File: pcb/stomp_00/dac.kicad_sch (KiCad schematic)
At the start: 6 parts, among them J4 Headphones, U9 SGTL5000XNAA3

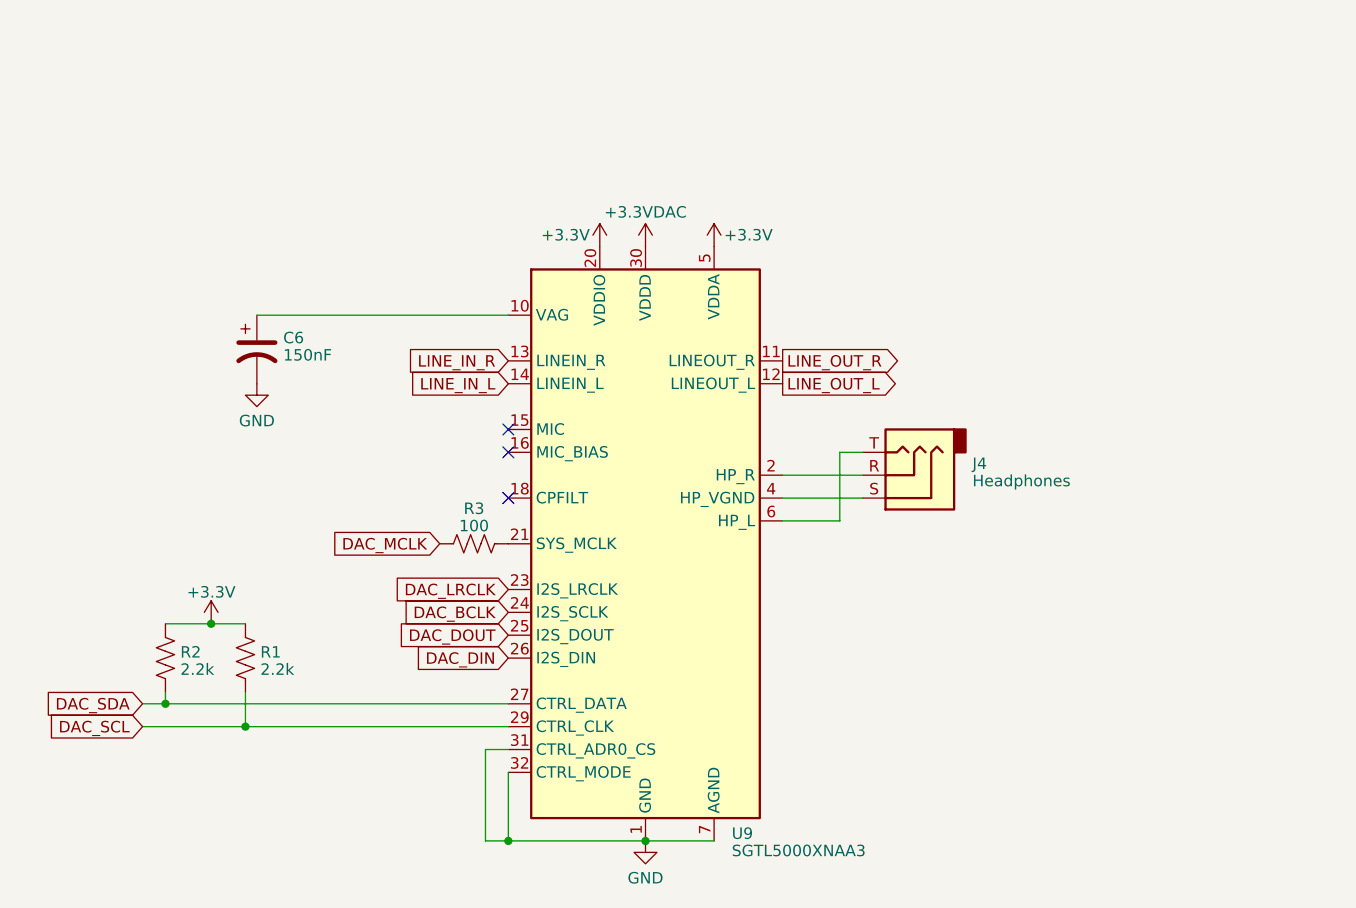
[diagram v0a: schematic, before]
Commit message: more input stage faffing
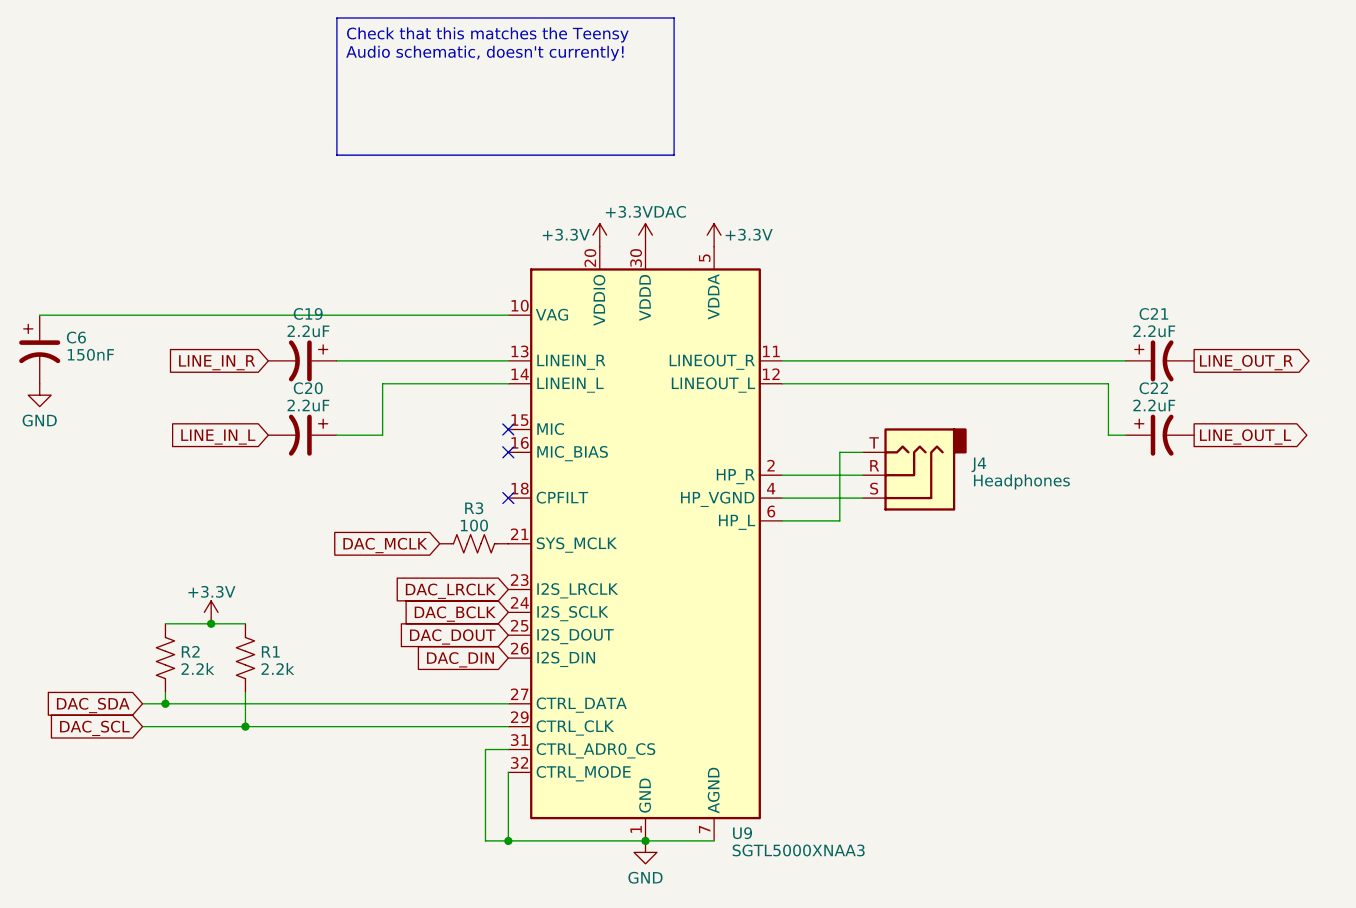
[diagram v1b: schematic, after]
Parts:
- added C19, C20, C21, C22: 2.2uF, symbol Device:C_Polarized_US
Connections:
- net LINE_IN_L: now also C20.2; no longer U9.14 (LINEIN_L)
- net LINE_IN_R: now also C19.2; no longer U9.13 (LINEIN_R)
- net LINE_OUT_L: now also C22.2; no longer U9.12 (LINEOUT_L)
- net LINE_OUT_R: now also C21.2; no longer U9.11 (LINEOUT_R)
- new net: C21.1, U9.11 (LINEOUT_R)
- new net: C22.1, U9.12 (LINEOUT_L)
- new net: C19.1, U9.13 (LINEIN_R)
- new net: C20.1, U9.14 (LINEIN_L)
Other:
- moved on the sheet: C6
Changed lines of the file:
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@@
+    (stroke (width 0) (type default))
+  )
+  (wire (pts (xy 160.02 73.66) (xy 198.12 73.66))
     (stroke (width 0) (type default))
   )
@@
     (stroke (width 0) (type default))
   )
+  (wire (pts (xy 110.49 81.915) (xy 115.57 81.915))
+    (stroke (width 0) (type default))
+  )
   (wire (pts (xy 100.33 110.49) (xy 100.33 114.3))
     (stroke (width 0) (type default))
@@
     (stroke (width 0) (type default))
   )
+  (wire (pts (xy 110.49 73.66) (xy 129.54 73.66))
+    (stroke (width 0) (type default))
+  )
   (wire (pts (xy 160.02 91.44) (xy 166.37 91.44))
     (stroke (width 0) (type default))
@@
     (stroke (width 0) (type default))
   )
-  (wire (pts (xy 101.6 68.58) (xy 129.54 68.58))
+  (wire (pts (xy 115.57 76.2) (xy 129.54 76.2))
+    (stroke (width 0) (type default))
+  )
+  (wire (pts (xy 77.47 68.58) (xy 129.54 68.58))
     (stroke (width 0) (type default))
   )
@@
     (stroke (width 0) (type default))
   )
+  (wire (pts (xy 196.215 76.2) (xy 196.215 81.915))
+    (stroke (width 0) (type default))
+  )
+  (wire (pts (xy 160.02 76.2) (xy 196.215 76.2))
+    (stroke (width 0) (type default))
+  )
+  (wire (pts (xy 115.57 76.2) (xy 115.57 81.915))
+    (stroke (width 0) (type default))
+  )
   (wire (pts (xy 166.37 83.82) (xy 168.91 83.82))
     (stroke (width 0) (type default))
@@
     (stroke (width 0) (type default))
   )
+  (wire (pts (xy 196.215 81.915) (xy 198.12 81.915))
+    (stroke (width 0) (type default))
+  )
   (wire (pts (xy 88.9 114.3) (xy 100.33 114.3))
     (stroke (width 0) (type default))
@@
     (stroke (width 0) (type default))
   )
-  (global_label "LINE_OUT_L" (shape output) (at 160.02 76.2 0) (fields_autoplaced)
+  (text_box "Check that this matches the Teensy Audio schematic, doesn't currently!"
+    (at 110.49 35.56 0) (size 37.465 15.24)
+    (stroke (width 0) (type default))
+    (fill (type none))
+    (effects (font (size 1.27 1.27)) (justify left top))
+  )
+  (global_label "LINE_OUT_L" (shape output) (at 205.74 81.915 0) (fields_autoplaced)
     (effects (font (size 1.27 1.27)) (justify left))
-    (property "Intersheetrefs" "${INTERSHEET_REFS}" (at 173.6301 76.2 0)
+    (property "Intersheetrefs" "${INTERSHEET_REFS}" (at 219.3501 81.915 0)
       (effects (font (size 1.27 1.27)) (justify left) hide)
     )
@@
     )
   )
-  (global_label "LINE_OUT_R" (shape output) (at 160.02 73.66 0) (fields_autoplaced)
+  (global_label "LINE_OUT_R" (shape output) (at 205.74 73.66 0) (fields_autoplaced)
     (effects (font (size 1.27 1.27)) (justify left))
-    (property "Intersheetrefs" "${INTERSHEET_REFS}" (at 173.872 73.66 0)
+    (property "Intersheetrefs" "${INTERSHEET_REFS}" (at 219.592 73.66 0)
       (effects (font (size 1.27 1.27)) (justify left) hide)
     )
   )
-  (global_label "LINE_IN_R" (shape input) (at 129.54 73.66 180) (fields_autoplaced)
-    (effects (font (size 1.27 1.27)) (justify right))
-    (property "Intersheetrefs" "${INTERSHEET_REFS}" (at 117.3813 73.66 0)
+  (global_label "LINE_IN_R" (shape input) (at 102.87 73.66 180) (fields_autoplaced)
+    (effects (font (size 1.27 1.27)) (justify right))
+    (property "Intersheetrefs" "${INTERSHEET_REFS}" (at 90.7113 73.66 0)
       (effects (font (size 1.27 1.27)) (justify right) hide)
     )
@@
     )
   )
-  (global_label "LINE_IN_L" (shape input) (at 129.54 76.2 180) (fields_autoplaced)
-    (effects (font (size 1.27 1.27)) (justify right))
-    (property "Intersheetrefs" "${INTERSHEET_REFS}" (at 117.6232 76.2 0)
+  (global_label "LINE_IN_L" (shape input) (at 102.87 81.915 180) (fields_autoplaced)
+    (effects (font (size 1.27 1.27)) (justify right))
+    (property "Intersheetrefs" "${INTERSHEET_REFS}" (at 90.9532 81.915 0)
       (effects (font (size 1.27 1.27)) (justify right) hide)
     )
@@
     )
   )
-  (symbol (lib_id "Device:C_Polarized_US") (at 101.6 72.39 0) (unit 1)
-    (in_bom yes) (on_board yes) (dnp no) (fields_autoplaced)
-    (property "Reference" "C6" (at 104.521 71.1113 0)
+  (symbol (lib_id "Device:C_Polarized_US") (at 77.47 72.39 0) (unit 1)
+    (in_bom yes) (on_board yes) (dnp no) (fields_autoplaced)
+    (property "Reference" "C6" (at 80.391 71.1113 0)
       (effects (font (size 1.27 1.27)) (justify left))
     )
-    (property "Value" "150nF" (at 104.521 73.0323 0)
+    (property "Value" "150nF" (at 80.391 73.0323 0)
       (effects (font (size 1.27 1.27)) (justify left))
     )
-    (property "Footprint" "" (at 101.6 72.39 0)
-      (effects (font (size 1.27 1.27)) hide)
-    )
-    (property "Datasheet" "~" (at 101.6 72.39 0)
+    (property "Footprint" "" (at 77.47 72.39 0)
+      (effects (font (size 1.27 1.27)) hide)
+    )
+    (property "Datasheet" "~" (at 77.47 72.39 0)
       (effects (font (size 1.27 1.27)) hide)
     )
@@
         (path "/8f4a2eb0-078b-46cb-b534-a4acd11d130e/7598c0f0-0137-4b50-80b5-b929d25c284a"
           (reference "C6") (unit 1)
+        )
+      )
+    )
+  )
+  (symbol (lib_id "Device:C_Polarized_US") (at 106.68 81.915 270) (unit 1)
+    (in_bom yes) (on_board yes) (dnp no) (fields_autoplaced)
+    (property "Reference" "C20" (at 107.315 76.7461 90)
+      (effects (font (size 1.27 1.27)))
+    )
+    (property "Value" "2.2uF" (at 107.315 78.6671 90)
+      (effects (font (size 1.27 1.27)))
+    )
+    (property "Footprint" "" (at 106.68 81.915 0)
+      (effects (font (size 1.27 1.27)) hide)
+    )
+    (property "Datasheet" "~" (at 106.68 81.915 0)
+      (effects (font (size 1.27 1.27)) hide)
+    )
+    (pin "1")
+    (pin "2")
+    (instances
+      (project "stomp_00"
+        (path "/8f4a2eb0-078b-46cb-b534-a4acd11d130e/7598c0f0-0137-4b50-80b5-b929d25c284a"
+          (reference "C20") (unit 1)
+        )
+      )
+    )
+  )
+  (symbol (lib_id "Device:C_Polarized_US") (at 201.93 73.66 90) (mirror x) (unit 1)
+    (in_bom yes) (on_board yes) (dnp no) (fields_autoplaced)
+    (property "Reference" "C21" (at 201.295 68.4911 90)
+      (effects (font (size 1.27 1.27)))
+    )
+    (property "Value" "2.2uF" (at 201.295 70.4121 90)
+      (effects (font (size 1.27 1.27)))
+    )
+    (property "Footprint" "" (at 201.93 73.66 0)
+      (effects (font (size 1.27 1.27)) hide)
+    )
+    (property "Datasheet" "~" (at 201.93 73.66 0)
+      (effects (font (size 1.27 1.27)) hide)
+    )
+    (pin "1")
+    (pin "2")
+    (instances
+      (project "stomp_00"
+        (path "/8f4a2eb0-078b-46cb-b534-a4acd11d130e/7598c0f0-0137-4b50-80b5-b929d25c284a"
+          (reference "C21") (unit 1)
         )
       )
@@
     )
   )
-  (symbol (lib_id "power:GND") (at 101.6 76.2 0) (unit 1)
-    (in_bom yes) (on_board yes) (dnp no) (fields_autoplaced)
-    (property "Reference" "#PWR011" (at 101.6 82.55 0)
-      (effects (font (size 1.27 1.27)) hide)
-    )
-    (property "Value" "GND" (at 101.6 80.3355 0)
-      (effects (font (size 1.27 1.27)))
-    )
-    (property "Footprint" "" (at 101.6 76.2 0)
-      (effects (font (size 1.27 1.27)) hide)
-    )
-    (property "Datasheet" "" (at 101.6 76.2 0)
+  (symbol (lib_id "power:GND") (at 77.47 76.2 0) (unit 1)
+    (in_bom yes) (on_board yes) (dnp no) (fields_autoplaced)
+    (property "Reference" "#PWR011" (at 77.47 82.55 0)
+      (effects (font (size 1.27 1.27)) hide)
+    )
+    (property "Value" "GND" (at 77.47 80.3355 0)
+      (effects (font (size 1.27 1.27)))
+    )
+    (property "Footprint" "" (at 77.47 76.2 0)
+      (effects (font (size 1.27 1.27)) hide)
+    )
+    (property "Datasheet" "" (at 77.47 76.2 0)
       (effects (font (size 1.27 1.27)) hide)
     )
@@
         (path "/8f4a2eb0-078b-46cb-b534-a4acd11d130e/7598c0f0-0137-4b50-80b5-b929d25c284a"
           (reference "R2") (unit 1)
+        )
+      )
+    )
+  )
+  (symbol (lib_id "Device:C_Polarized_US") (at 201.93 81.915 90) (mirror x) (unit 1)
+    (in_bom yes) (on_board yes) (dnp no) (fields_autoplaced)
+    (property "Reference" "C22" (at 201.295 76.7461 90)
+      (effects (font (size 1.27 1.27)))
+    )
+    (property "Value" "2.2uF" (at 201.295 78.6671 90)
+      (effects (font (size 1.27 1.27)))
+    )
+    (property "Footprint" "" (at 201.93 81.915 0)
+      (effects (font (size 1.27 1.27)) hide)
+    )
+    (property "Datasheet" "~" (at 201.93 81.915 0)
+      (effects (font (size 1.27 1.27)) hide)
+    )
+    (pin "1")
+    (pin "2")
+    (instances
+      (project "stomp_00"
+        (path "/8f4a2eb0-078b-46cb-b534-a4acd11d130e/7598c0f0-0137-4b50-80b5-b929d25c284a"
+          (reference "C22") (unit 1)
         )
       )
@@
         )
       )
+    )
+  )
+  (symbol (lib_id "Device:C_Polarized_US") (at 106.68 73.66 270) (unit 1)
+    (in_bom yes) (on_board yes) (dnp no) (fields_autoplaced)
+    (property "Reference" "C19" (at 107.315 68.4911 90)
+      (effects (font (size 1.27 1.27)))
+    )
+    (property "Value" "2.2uF" (at 107.315 70.4121 90)
+      (effects (font (size 1.27 1.27)))
+    )
+    (property "Footprint" "" (at 106.68 73.66 0)
+      (effects (font (size 1.27 1.27)) hide)
+    )
+    (property "Datasheet" "~" (at 106.68 73.66 0)
+      (effects (font (size 1.27 1.27)) hide)
+    )
+    (pin "1")
+    (pin "2")
+    (instances
+      (project "stomp_00"
+        (path "/8f4a2eb0-078b-46cb-b534-a4acd11d130e/7598c0f0-0137-4b50-80b5-b929d25c284a"
+          (reference "C19") (unit 1)
+        )
+      )
